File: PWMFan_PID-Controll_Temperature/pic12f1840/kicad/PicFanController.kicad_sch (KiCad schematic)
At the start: 10 parts, among them M2 Fan_4pin, SW1 2MS1-T1-B4-M2-Q-E, U1 MCP9700Ax-ETT, U1 PIC12F1840-IP

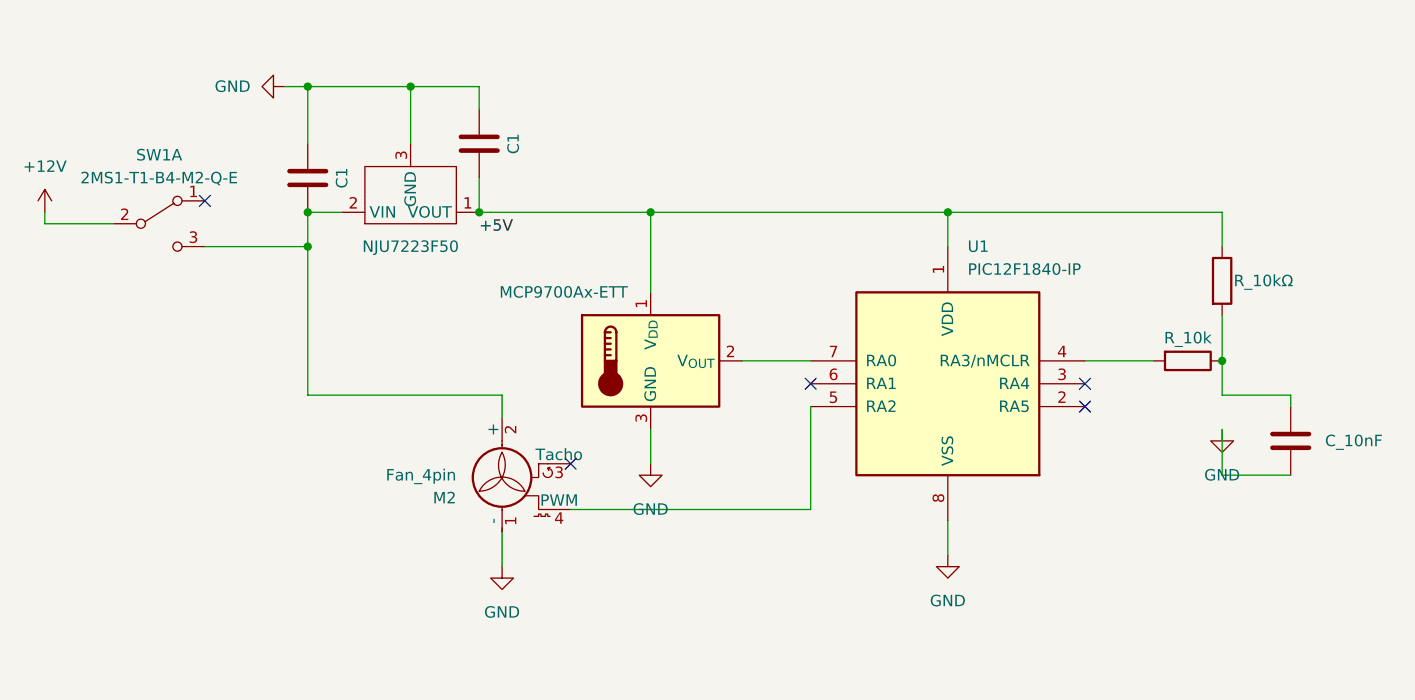
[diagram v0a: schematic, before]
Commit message: update
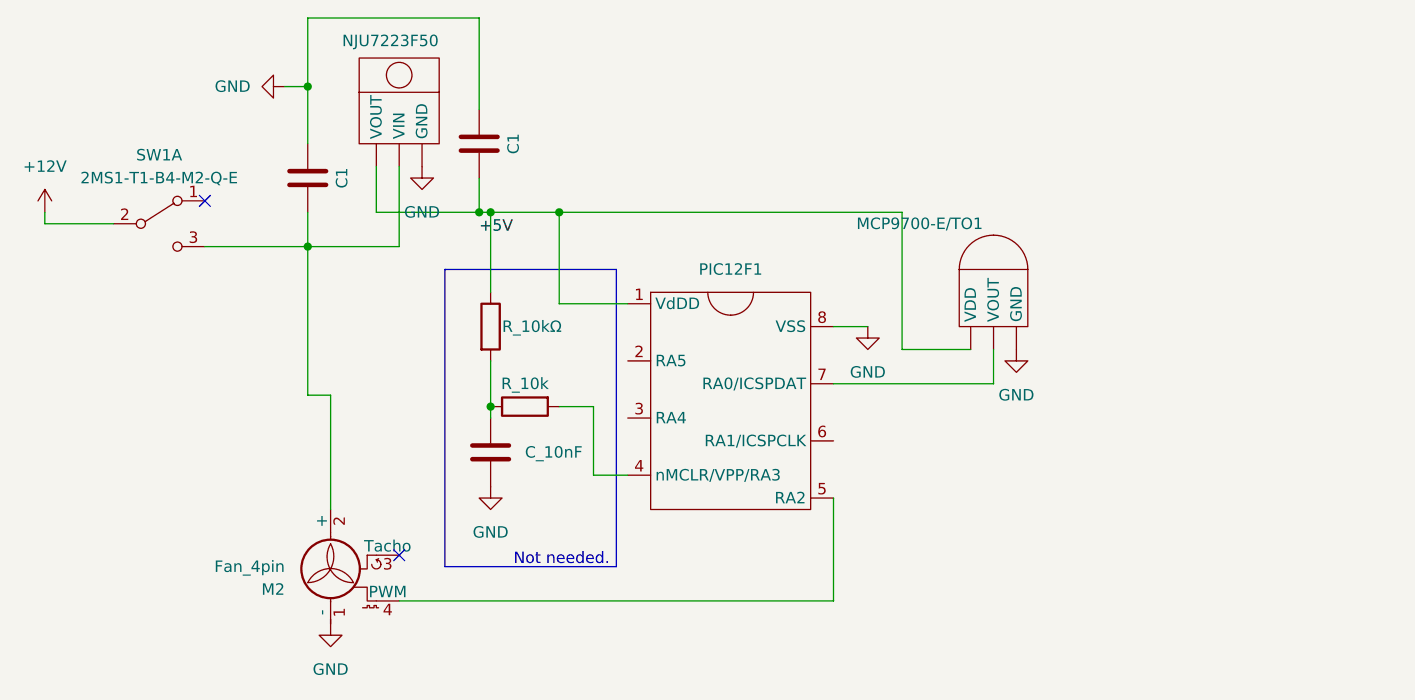
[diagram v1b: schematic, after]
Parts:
- removed U1: MCP9700Ax-ETT, Package_TO_SOT_SMD:SOT-23, symbol Sensor_Temperature:MCP9700Ax-ETT
- removed U1: PIC12F1840-IP, Package_DIP:DIP-8_W7.62mm, symbol MCU_Microchip_PIC12:PIC12F1840-IP
- added MCP9700-E/TO1: ~, symbol Ore:MCP9700-E/TO
- added PIC12F1: ~, symbol Ore:PIC12F1840
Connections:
- net GND: now also NJU7223F50. (VOUT), MCP9700-E/TO1. (VOUT), PIC12F1.8 (VSS); no longer NJU7223F50.3 (GND)
- net at C1.1, R_10kΩ.1: now also NJU7223F50. (VOUT), MCP9700-E/TO1. (VOUT), PIC12F1.1 (VdDD); no longer NJU7223F50.1 (VOUT)
- net at C1.1, M2.2 (+), SW1.3 (C): now also NJU7223F50. (VOUT); no longer NJU7223F50.2 (VIN)
- net at R_10k.2: now also PIC12F1.4 (nMCLR/VPP/RA3)
- net at M2.4 (PWM): now also PIC12F1.5 (RA2)
- new net: MCP9700-E/TO1. (VOUT), PIC12F1.7 (RA0/ICSPDAT)
- no-connect marks 5 -> 2
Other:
- note added: "Not needed."
- moved on the sheet: C_10nF, M2, R_10k, R_10kΩ
